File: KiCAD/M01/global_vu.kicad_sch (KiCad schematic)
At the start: 66 parts, among them J1 Conn_01x05, J2 Conn_01x05, U1 SR1-ML, U2 SR2-ML, U3 SR1-MR, U4 SR2-MR

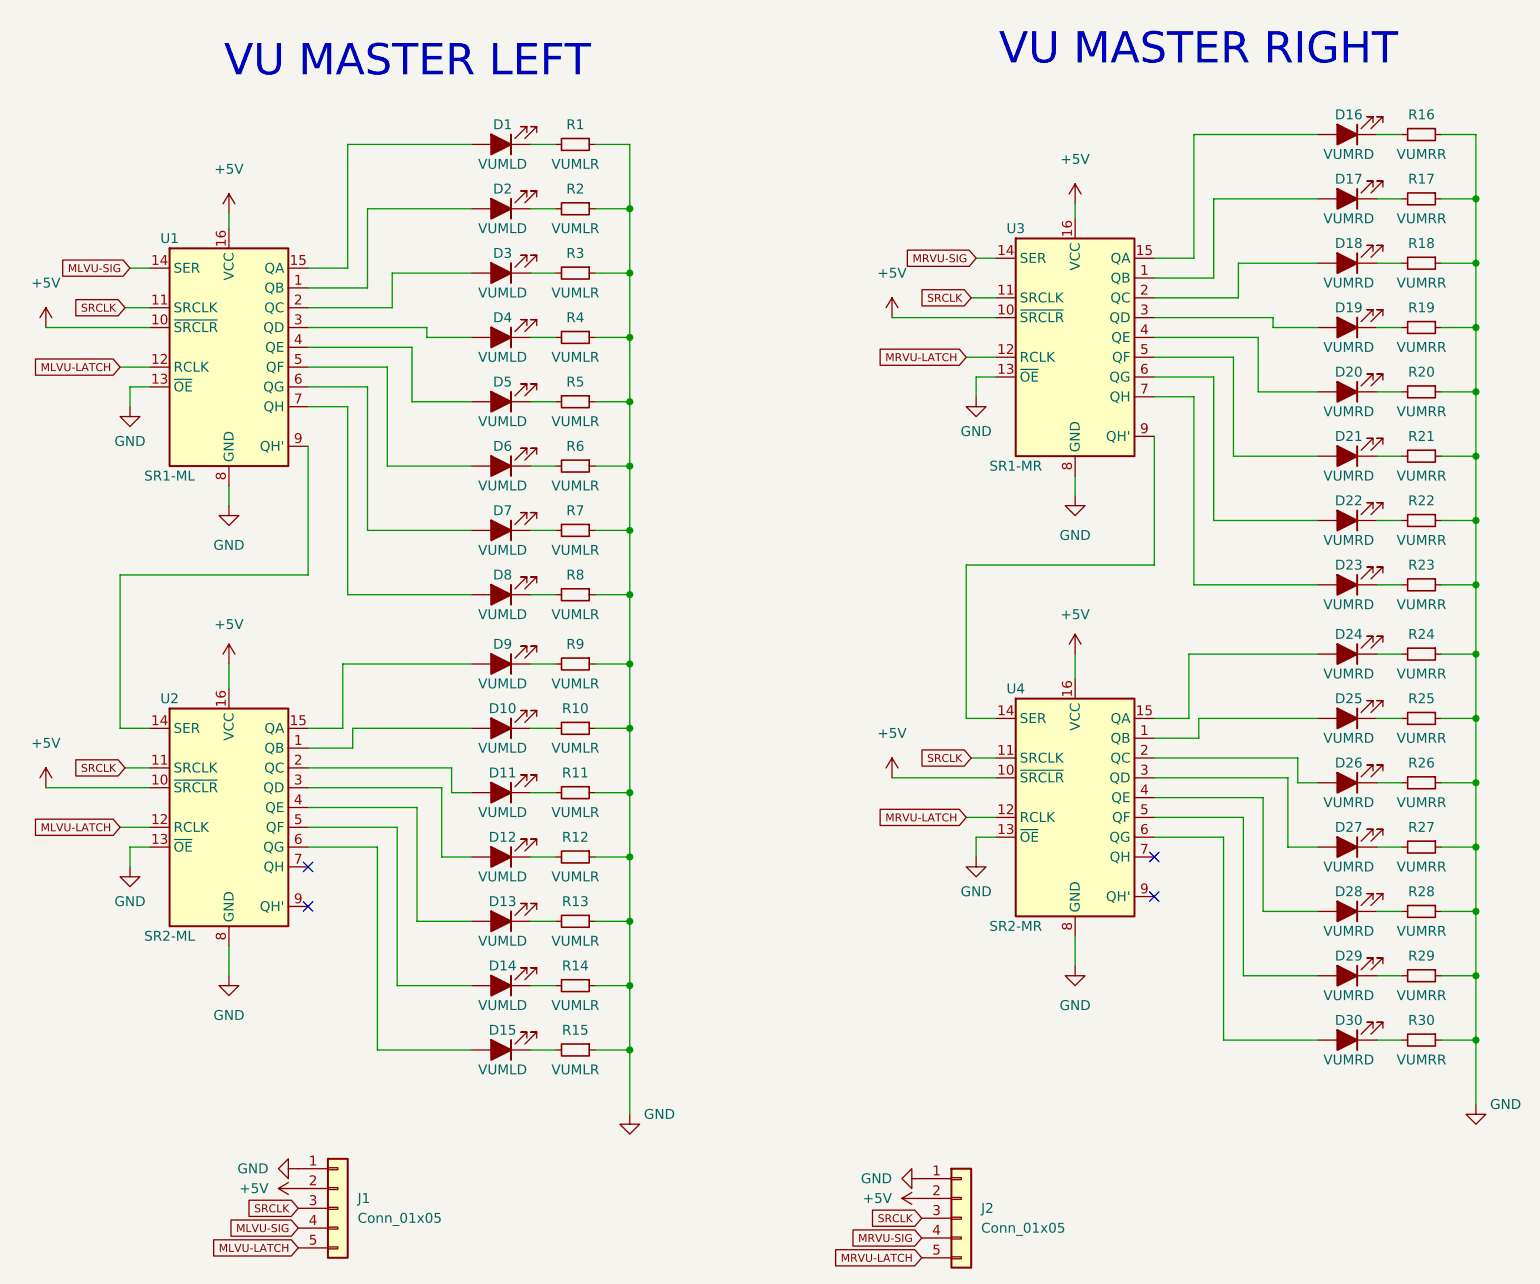
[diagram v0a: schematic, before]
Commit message: M01 fixes
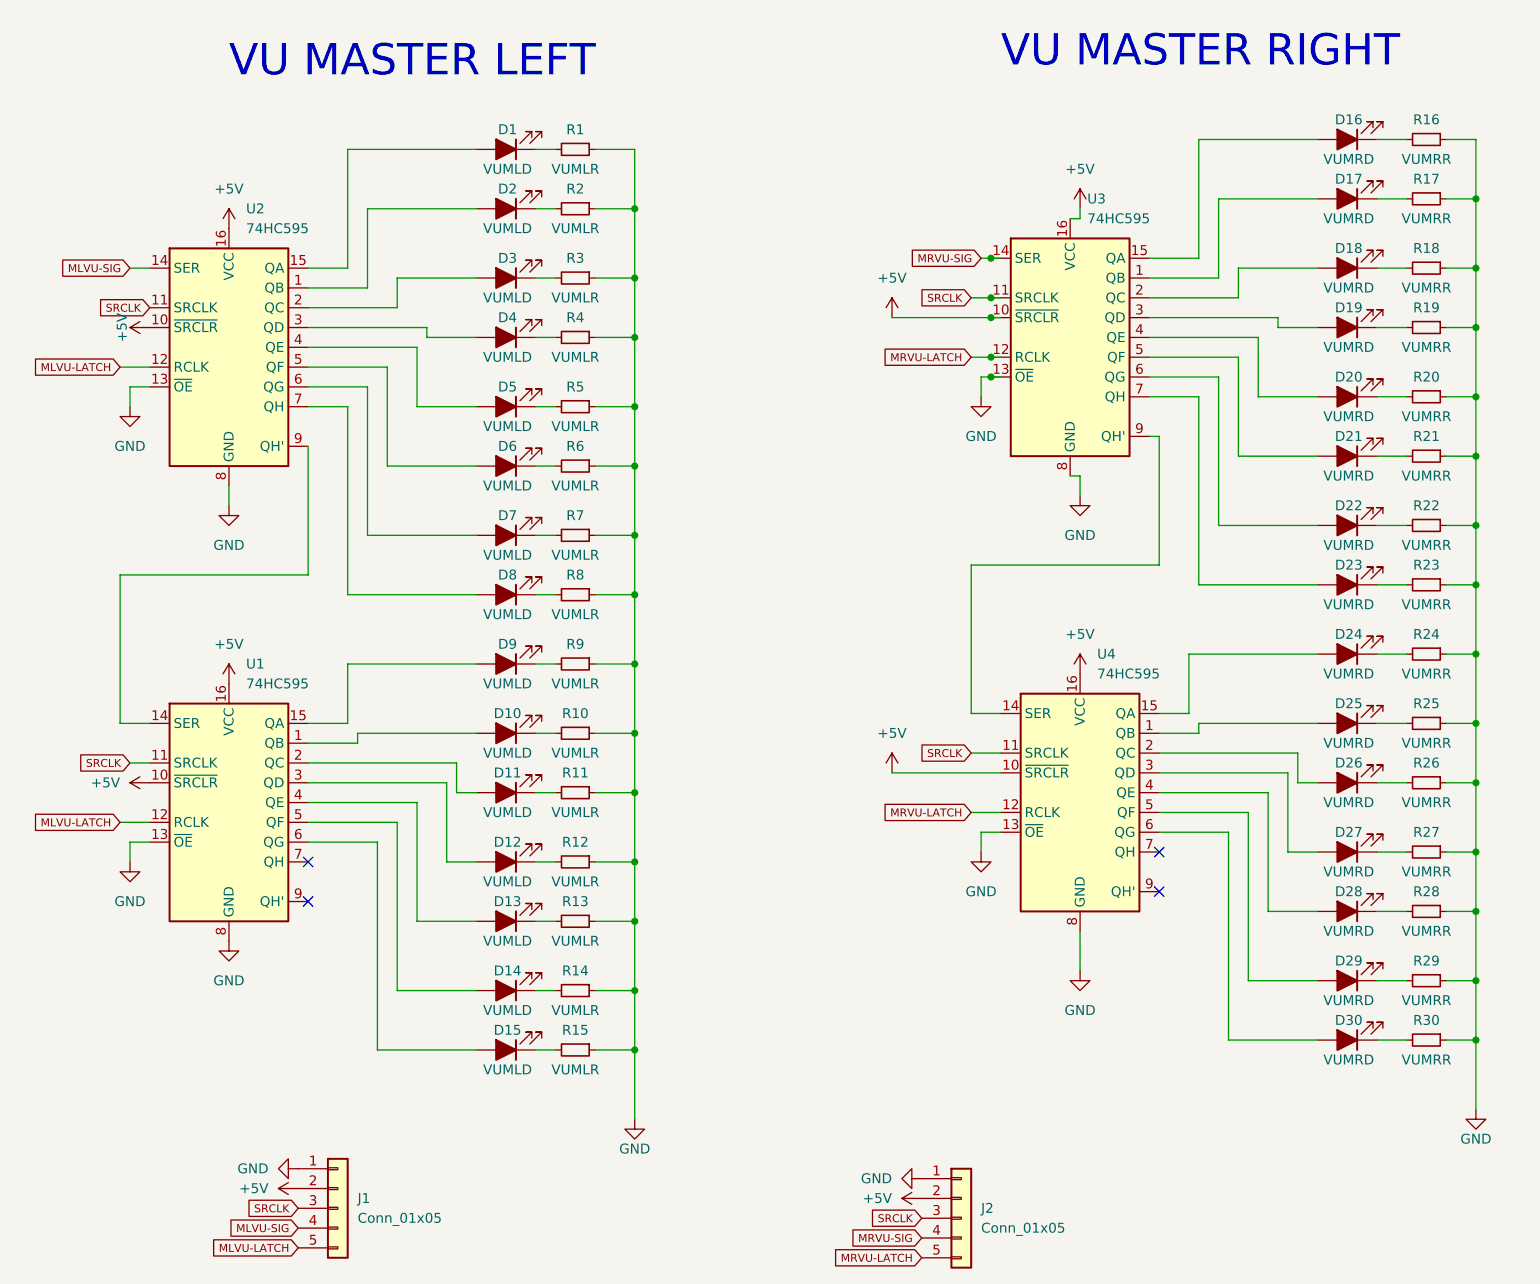
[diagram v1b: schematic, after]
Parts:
- D1, D16, D17, D2: footprint Library:LED_RED -> LED_THT:LED_D3.0mm
- D10, D11, D12, D13, D14, D15, D22, D23, D24, D25, D26, D27, D28, D29, D30, D7, D8, D9: footprint Library:LED_GREEN -> LED_THT:LED_D3.0mm
- D18, D19, D20, D21, D3, D4, D5, D6: footprint Library:LED_YELLOW -> LED_THT:LED_D3.0mm
- J1, J2: footprint (none) -> Connector_PinSocket_2.54mm:PinSocket_1x05_P2.54mm_Vertical
- U1: value SR1-ML -> 74HC595; footprint Package_SO:SOIC-16_3.9x9.9mm_P1.27mm -> Package_SO:SOIC-16W_5.3x10.2mm_P1.27mm
- U2: value SR2-ML -> 74HC595; footprint Package_SO:SOIC-16_3.9x9.9mm_P1.27mm -> Package_SO:SOIC-16W_5.3x10.2mm_P1.27mm
- U3: value SR1-MR -> 74HC595; footprint Package_SO:SOIC-16_3.9x9.9mm_P1.27mm -> Package_SO:SOIC-16W_5.3x10.2mm_P1.27mm
- U4: value SR2-MR -> 74HC595; footprint Package_SO:SOIC-16_3.9x9.9mm_P1.27mm -> Package_SO:SOIC-16W_5.3x10.2mm_P1.27mm
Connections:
- net MLVU-SIG: now also U2.14 (SER); no longer U1.14 (SER)
- net at U2.1 (QB): now also D2.2 (A); no longer D10.2 (A)
- net at U1.9 (QH'): no longer U2.14 (SER)
- net at U2.15 (QA): now also D1.2 (A); no longer D9.2 (A)
- net at U2.2 (QC): now also D3.2 (A); no longer D11.2 (A)
- net at U2.3 (QD): now also D4.2 (A); no longer D12.2 (A)
- net at U2.4 (QE): now also D5.2 (A); no longer D13.2 (A)
- net at U2.5 (QF): now also D6.2 (A); no longer D14.2 (A)
- net at U2.6 (QG): now also D7.2 (A); no longer D15.2 (A)
- net at U2.7 (QH): now also D8.2 (A)
- net at U2.9 (QH'): now also U1.14 (SER)
- net at U1.15 (QA): now also D9.2 (A); no longer D1.2 (A)
- net at U1.3 (QD): now also D12.2 (A); no longer D4.2 (A)
- net at U1.6 (QG): now also D15.2 (A); no longer D7.2 (A)
- net at U1.5 (QF): now also D14.2 (A); no longer D6.2 (A)
- net at U1.1 (QB): now also D10.2 (A); no longer D2.2 (A)
- net at U1.2 (QC): now also D11.2 (A); no longer D3.2 (A)
- net at U1.4 (QE): now also D13.2 (A); no longer D5.2 (A)
- net at U1.7 (QH): no longer D8.2 (A)
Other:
- moved on the sheet: D1, D10, D11, D12, D13, D14, D15, D16, D18, D2, D20, D22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
